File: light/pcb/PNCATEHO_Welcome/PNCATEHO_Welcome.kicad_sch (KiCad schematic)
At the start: 51 parts, among them J1 USB_C_Receptacle_USB2.0, SW11 Boot, SW12 Reset, U1 RP2040, U2 RT9013-33GB, U3 W25Q32JVSSIQ, U4 USBLC6-2SC6, Y1 12MHz

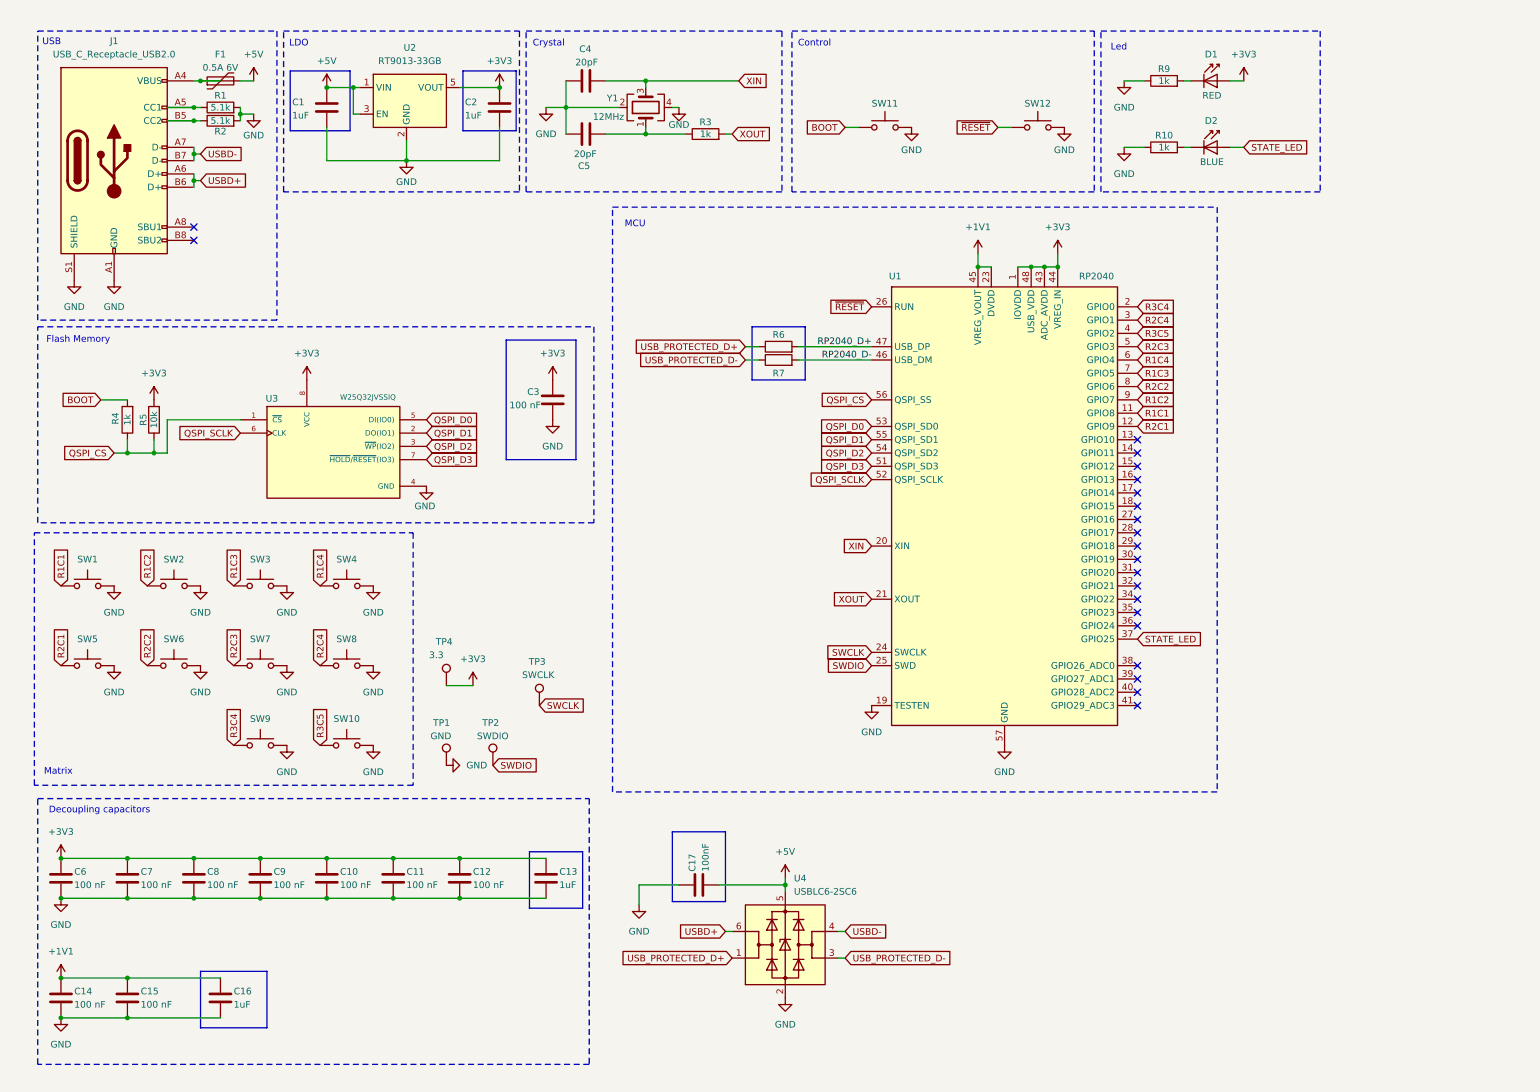
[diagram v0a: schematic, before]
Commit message: clear sch
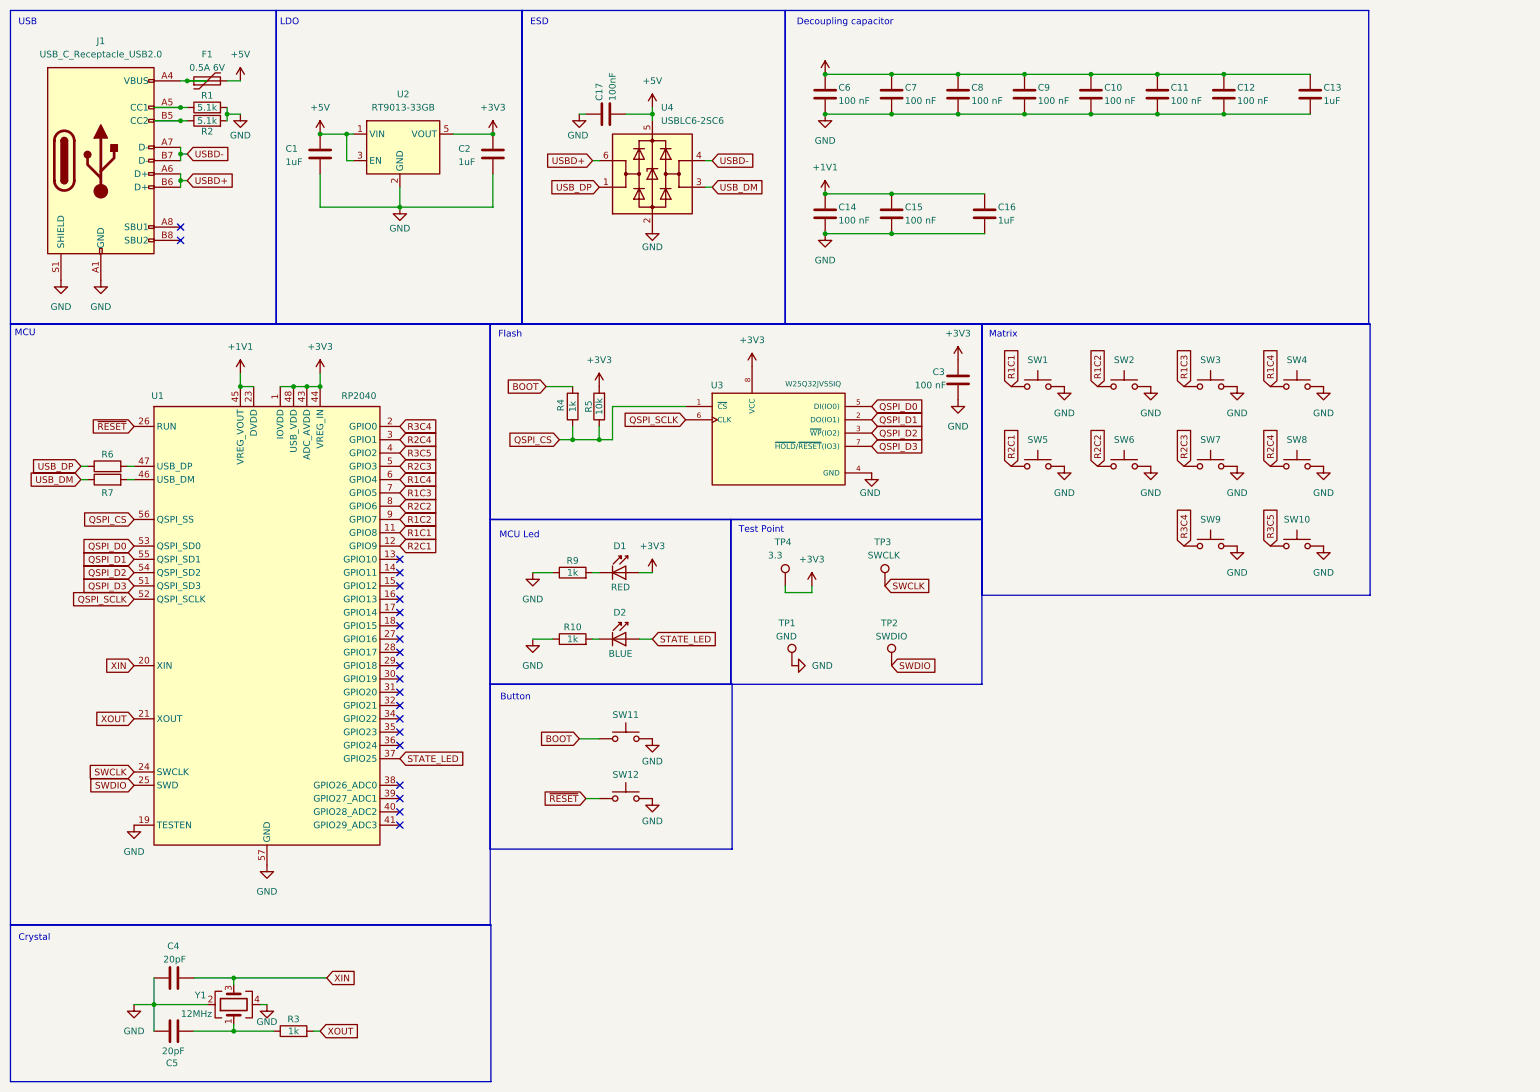
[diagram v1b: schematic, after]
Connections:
- net RP2040_D+: no longer names the net of R6.2, U1.47 (USB_DP)
- net RP2040_D-: no longer names the net of R7.2, U1.46 (USB_DM)
- net USB_PROTECTED_D+ renamed USB_DP
- net USB_PROTECTED_D- renamed USB_DM
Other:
- note added: "Button"
- note added: "Decoupling capacitor"
- note added: "ESD"
- note added: "Flash"
- note added: "MCU Led"
- note added: "Test Point"
- note removed: "Control"
- note removed: "Decoupling capacitors"
- note removed: "Flash Memory"
- note removed: "Led"
- moved on the sheet: C1, C10, C11, C12, C13, C14, C15, C16, C17, C2, C3, C4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

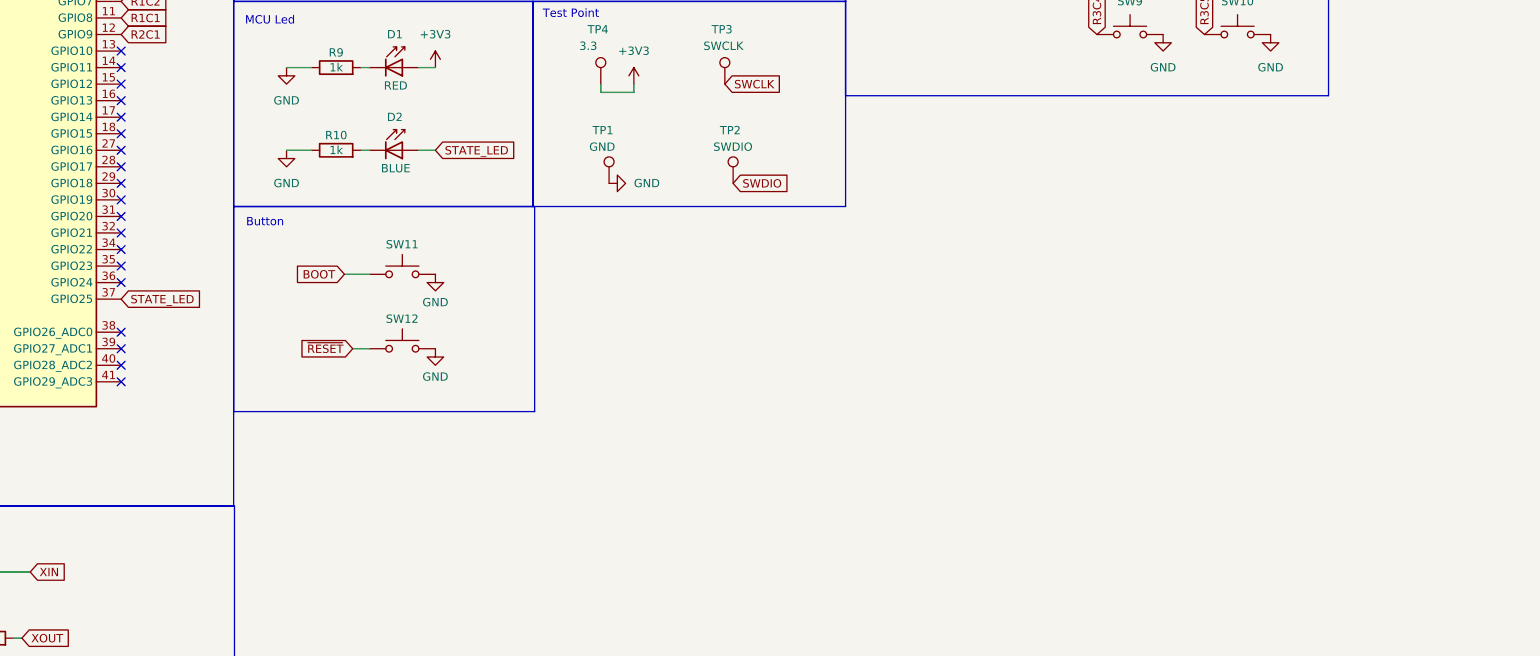
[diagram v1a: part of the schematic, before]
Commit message: add led
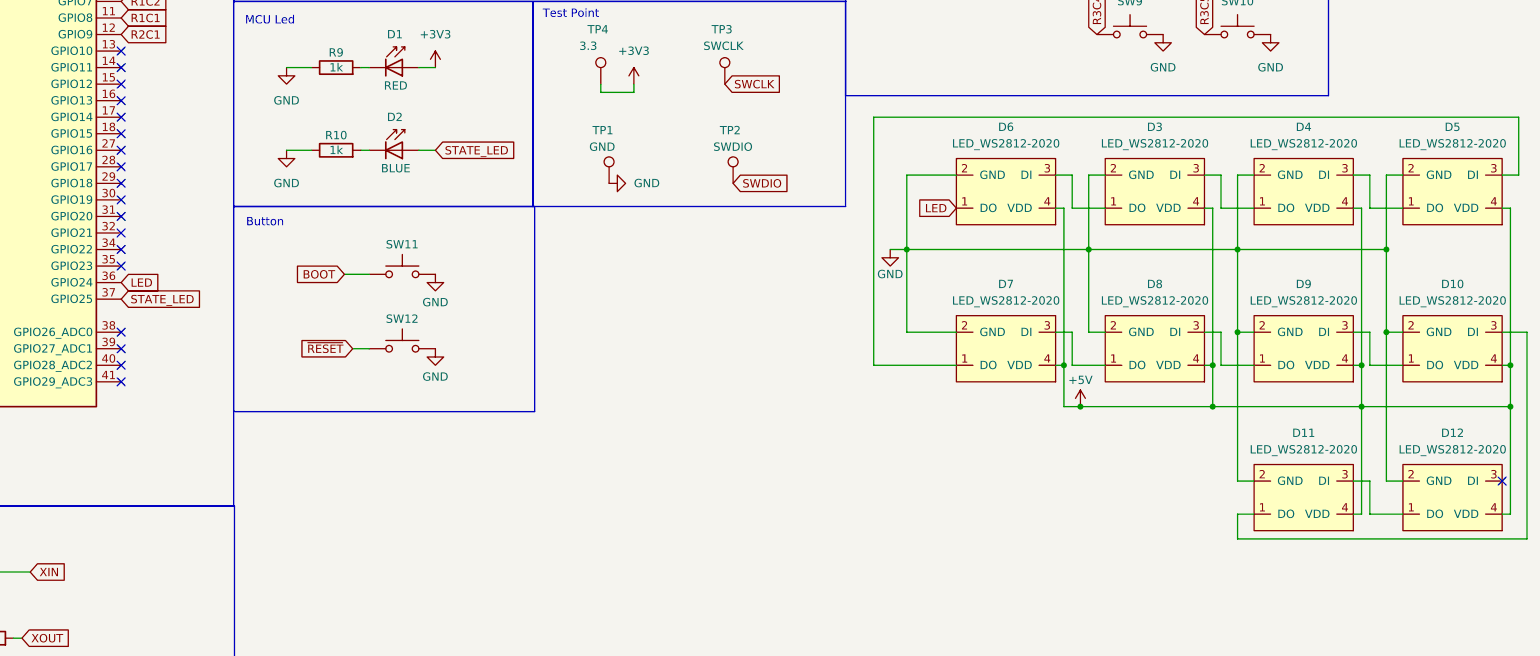
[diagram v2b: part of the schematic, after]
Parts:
- added D10, D11, D12, D3, D4, D5, D6, D7, D8, D9: LED_WS2812-2020, PNCATEHO:WS2812-2020-2.00mmx2.20mm, symbol ws2812:LED_WS2812-2020
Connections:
- net +5V: now also D10.4 (VDD), D11.4 (VDD), D12.4 (VDD), D3.4 (VDD), D4.4 (VDD), D5.4 (VDD), D6.4 (VDD), D7.4 (VDD), D8.4 (VDD), D9.4 (VDD)
- net GND: now also D10.2 (GND), D11.2 (GND), D12.2 (GND), D3.2 (GND), D4.2 (GND), D5.2 (GND), D6.2 (GND), D7.2 (GND), D8.2 (GND), D9.2 (GND)
- net LED: now reaches U1.36 (GPIO24)
- net LED: now also D6.1 (DO)
- new net: D3.1 (DO), D6.3 (DI)
- new net: D3.3 (DI), D4.1 (DO)
- new net: D4.3 (DI), D5.1 (DO)
- new net: D5.3 (DI), D7.1 (DO)
- new net: D10.3 (DI), D11.1 (DO)
- new net: D11.3 (DI), D12.1 (DO)
- new net: D10.1 (DO), D9.3 (DI)
- new net: D7.3 (DI), D8.1 (DO)
- new net: D8.3 (DI), D9.1 (DO)

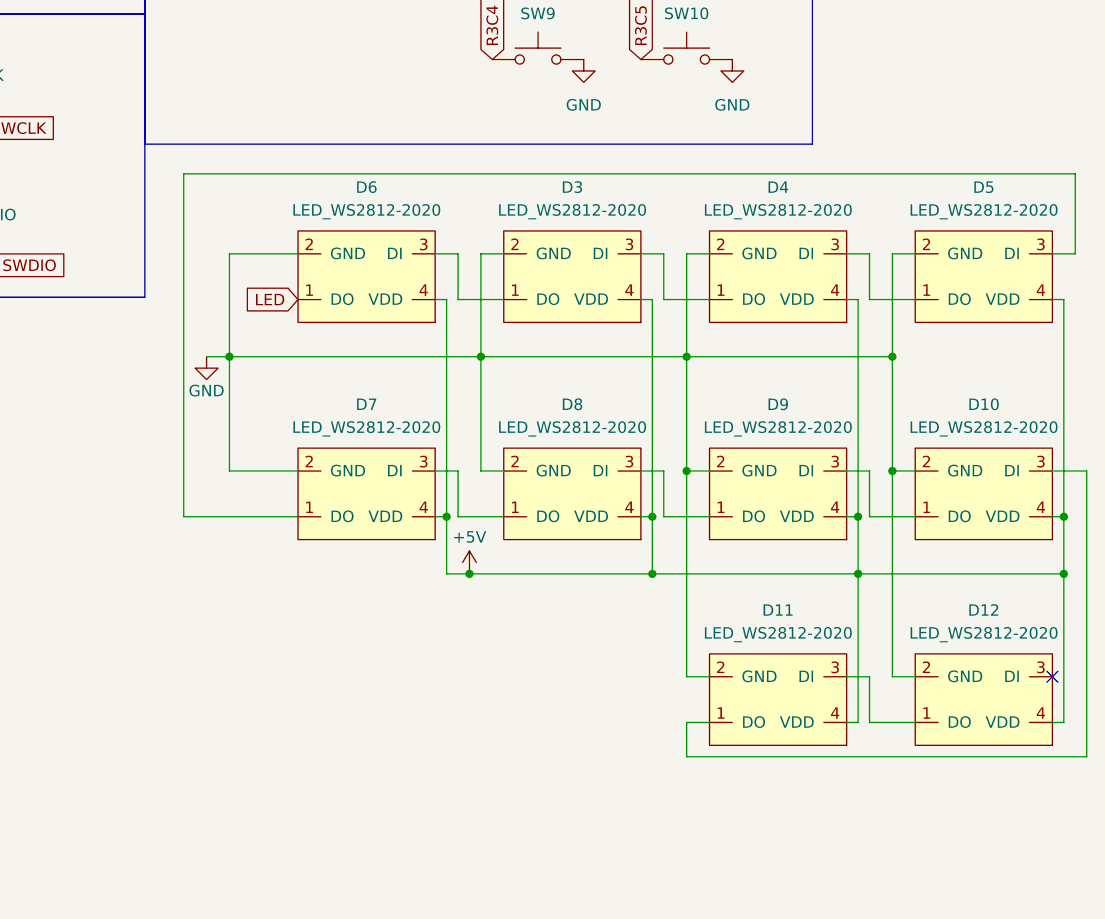
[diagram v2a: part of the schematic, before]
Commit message: fix sh
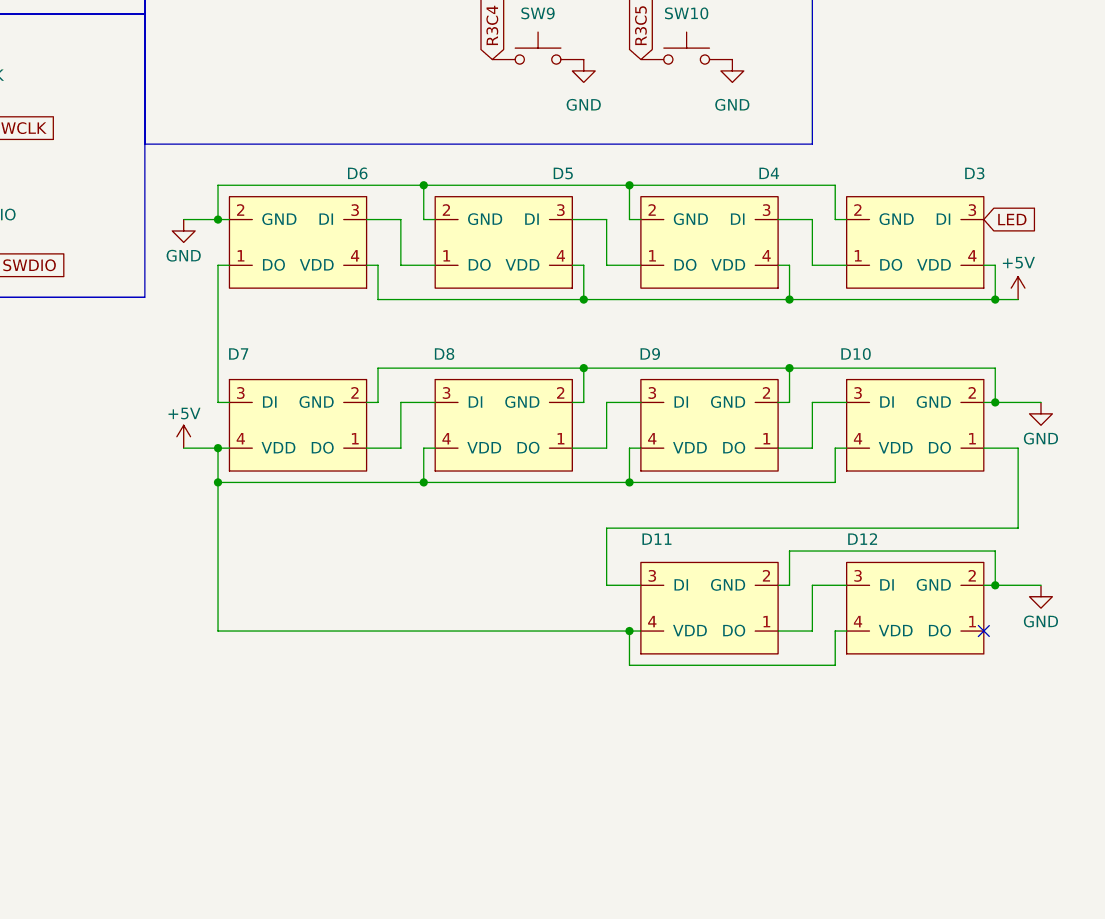
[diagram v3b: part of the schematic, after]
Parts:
- removed D10, D11, D12, D3, D4, D5, D6, D7, D8, D9: LED_WS2812-2020, PNCATEHO:WS2812-2020-2.00mmx2.20mm, symbol ws2812:LED_WS2812-2020
- added D10, D11, D12, D3, D4, D5, D6, D7, D8, D9: ~, PNCATEHO:WS2812-2020-2.00mmx2.20mm, symbol PNCATEHO:LED_WS2812-2020
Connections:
- net +5V: now also D10.4 (VDD), D11.4 (VDD), D12.4 (VDD), D3.4 (VDD), D4.4 (VDD), D5.4 (VDD), D6.4 (VDD), D7.4 (VDD), D8.4 (VDD), D9.4 (VDD)
- net GND: now also D10.2 (GND), D11.2 (GND), D12.2 (GND), D3.2 (GND), D4.2 (GND), D5.2 (GND), D6.2 (GND), D7.2 (GND), D8.2 (GND), D9.2 (GND)
- net LED: now also D3.3 (DI)
- new net: D8.1 (DO), D9.3 (DI)
- new net: D7.1 (DO), D8.3 (DI)
- new net: D5.1 (DO), D6.3 (DI)
- new net: D4.1 (DO), D5.3 (DI)
- new net: D6.1 (DO), D7.3 (DI)
- new net: D10.3 (DI), D9.1 (DO)
- new net: D3.1 (DO), D4.3 (DI)
- new net: D10.1 (DO), D11.3 (DI)
- new net: D11.1 (DO), D12.3 (DI)

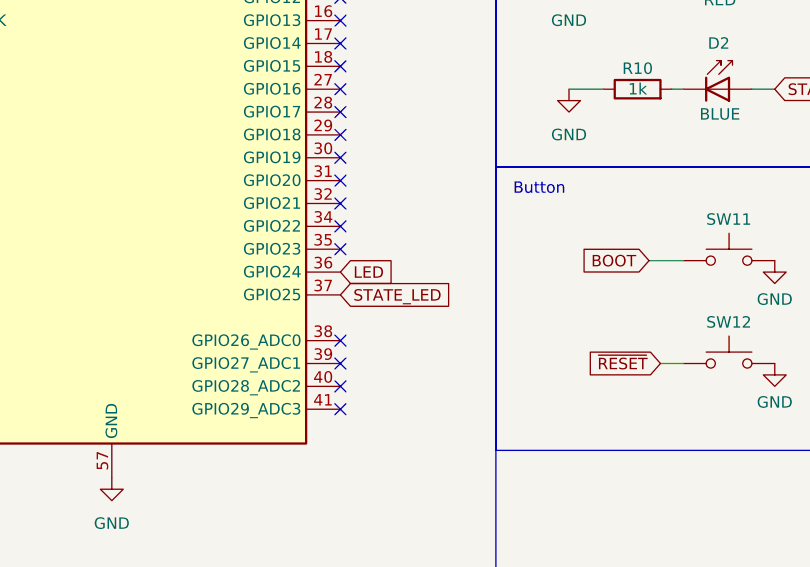
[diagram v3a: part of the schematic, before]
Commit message: PNCATEHO Welcome RGB routing
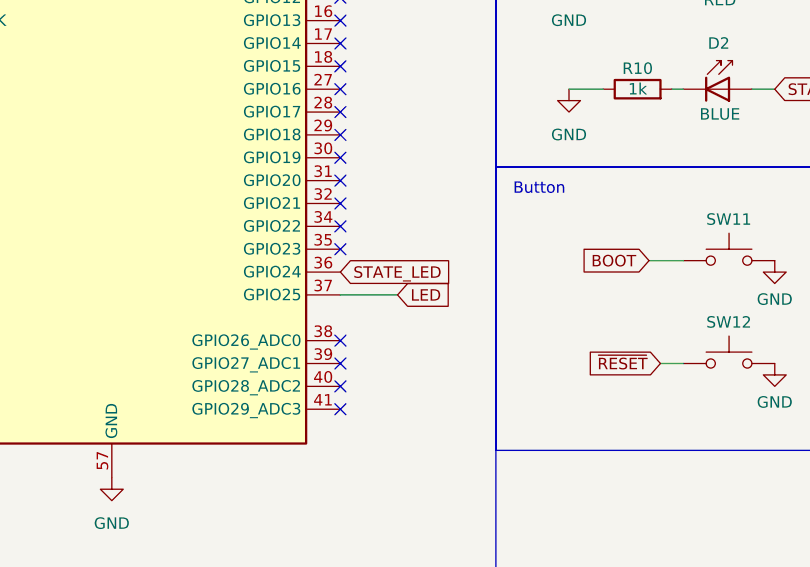
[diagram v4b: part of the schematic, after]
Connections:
- net LED: now also U1.37 (GPIO25); no longer U1.36 (GPIO24)
- net STATE_LED: now also U1.36 (GPIO24); no longer U1.37 (GPIO25)
